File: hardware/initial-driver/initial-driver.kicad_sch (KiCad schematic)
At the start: 10 parts, among them J1 PWR_IN, J2 MOTOR, J3 BREAK, J4 USB_C, U1 ESP32-S3-WROOM-1, U9 SN65HVD230

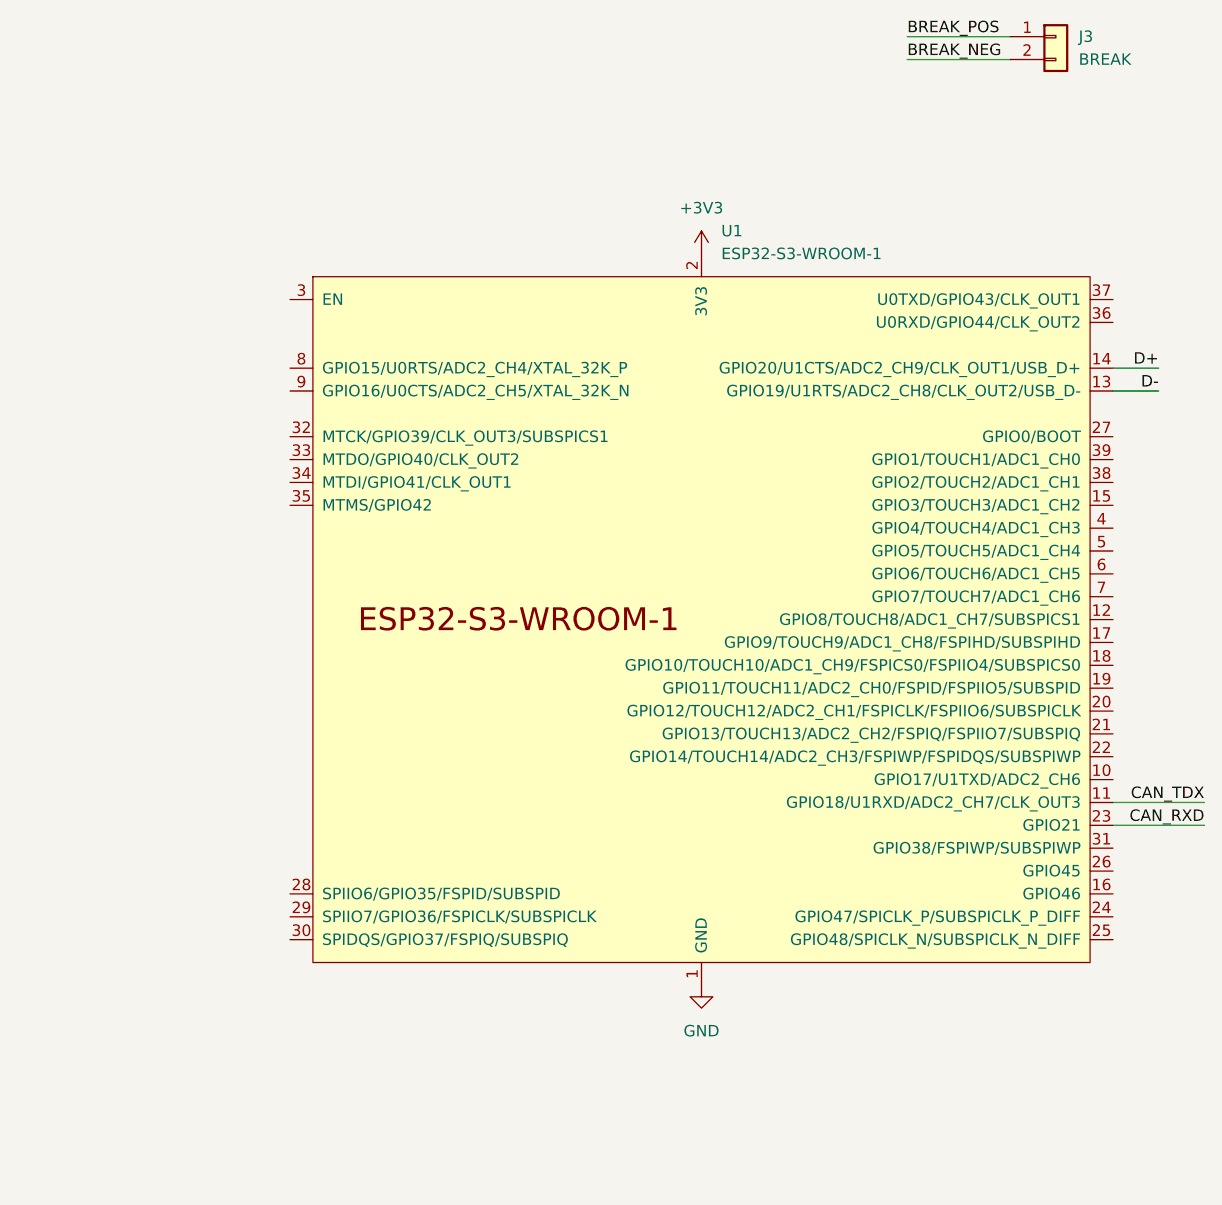
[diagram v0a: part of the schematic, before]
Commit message: add more stuff
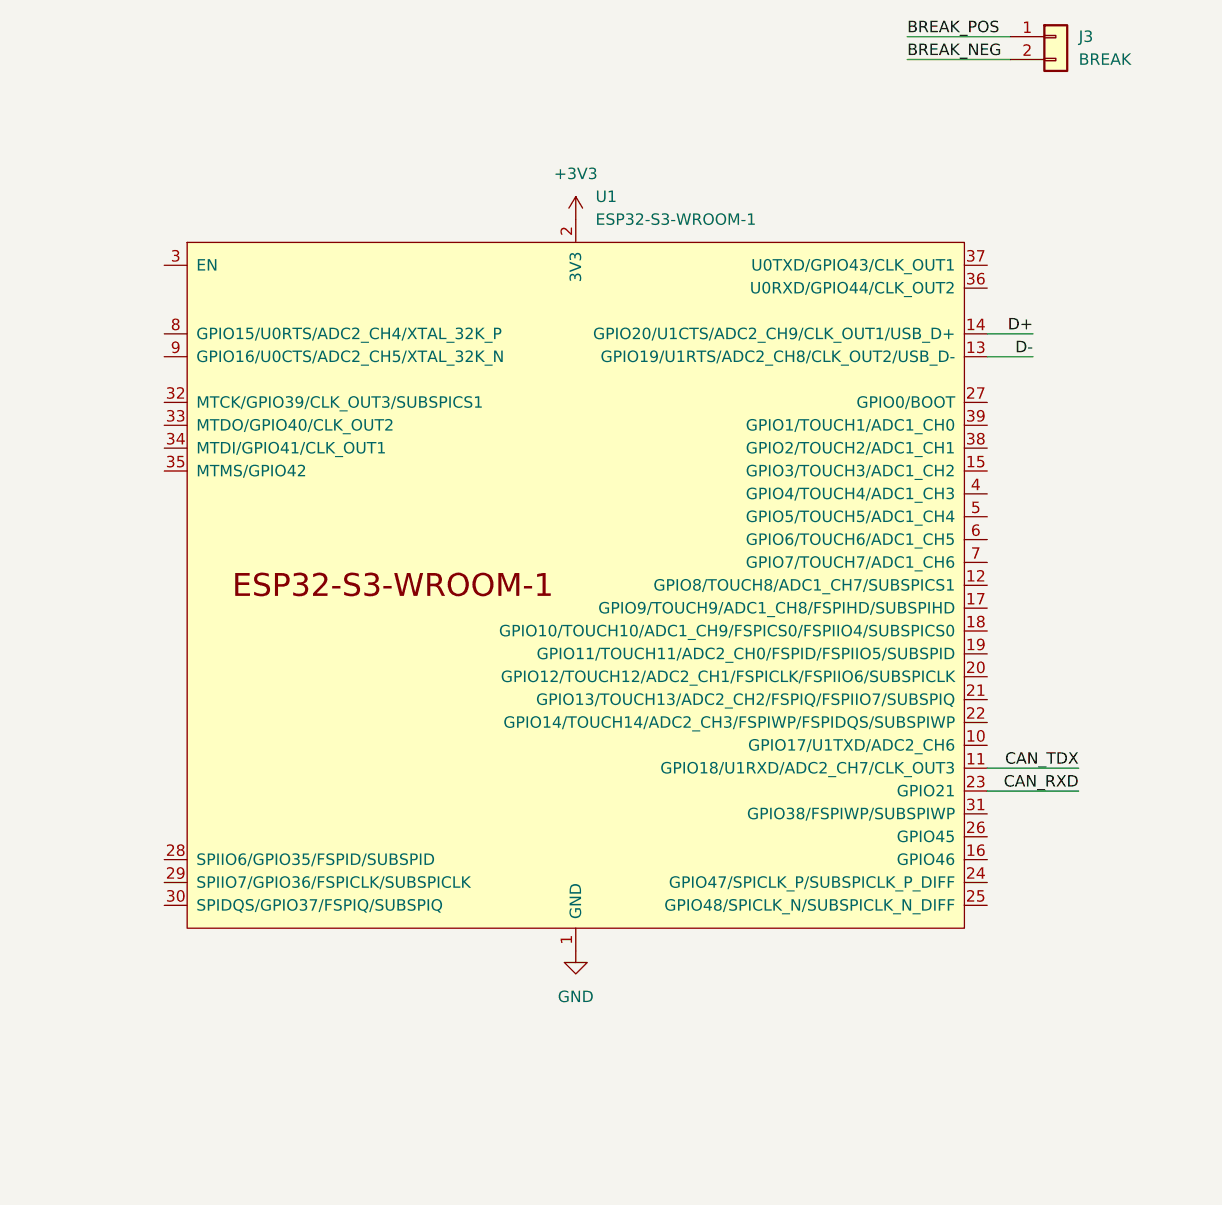
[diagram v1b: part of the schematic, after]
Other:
- moved on the sheet: U1
